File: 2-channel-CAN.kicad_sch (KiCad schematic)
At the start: 21 parts, among them K1 G6K-2 12V, Q1 PZT2222A, U6 MCP2515-xSO, U7 SN65HVD230, U8 SN65HVD230, Y2 8MHz

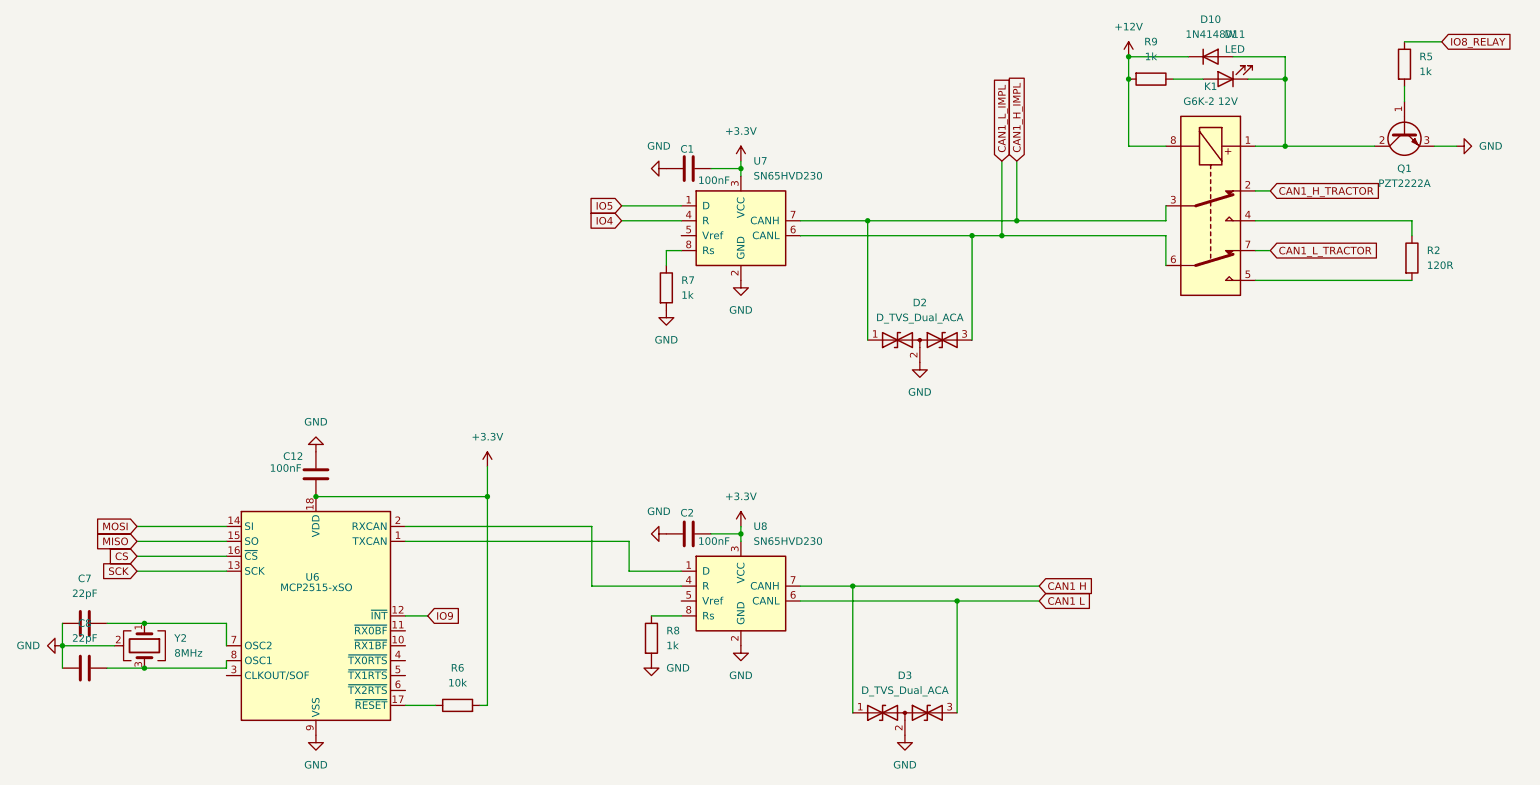
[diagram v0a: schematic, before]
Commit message: Fixes 20/10/2026
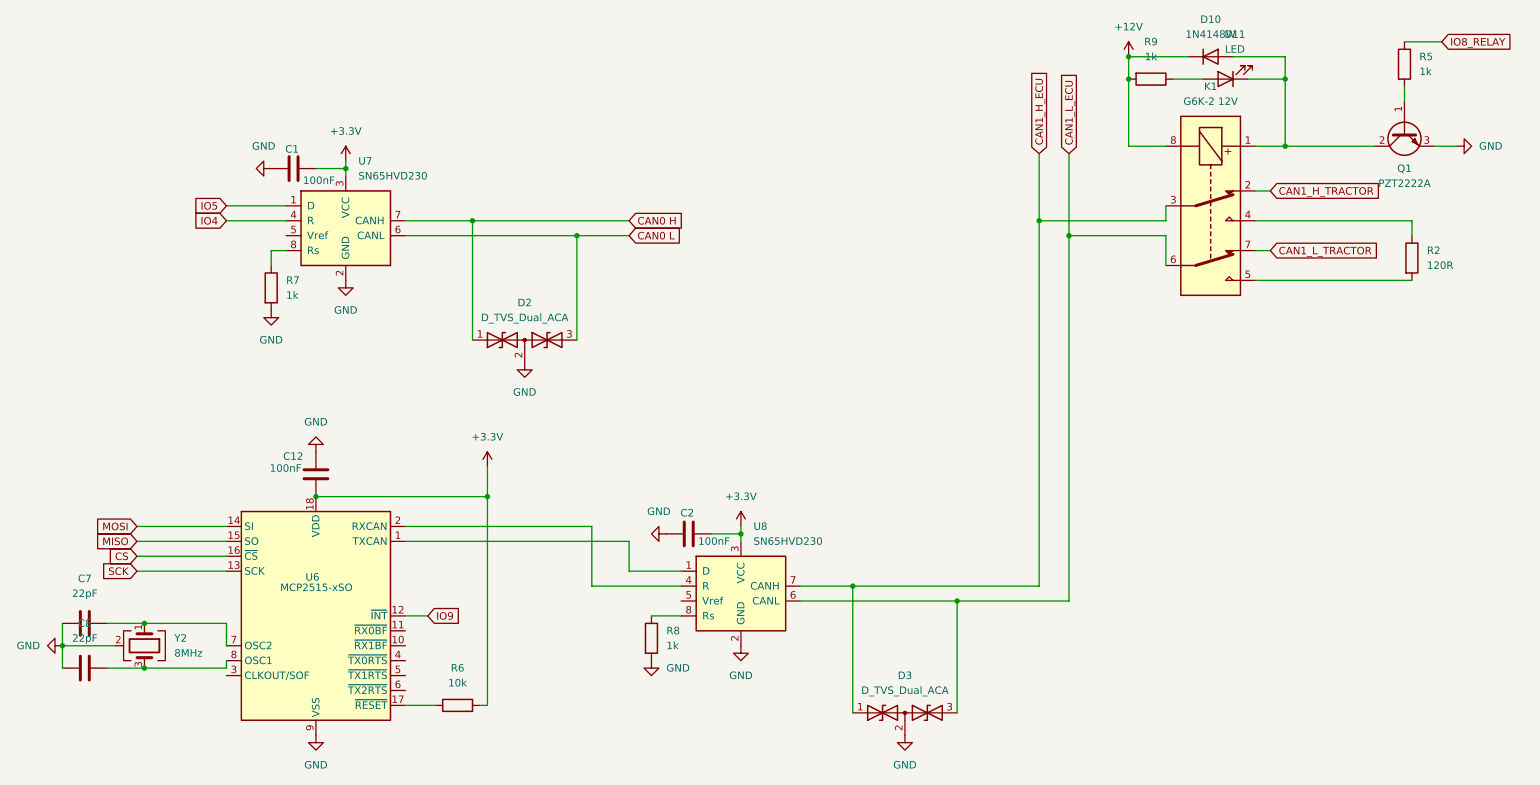
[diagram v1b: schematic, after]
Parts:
- D11: now in the parts list
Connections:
- net CAN1 H renamed CAN1_H_ECU
- net CAN1_H_ECU: now also K1.3
- net CAN1 L renamed CAN1_L_ECU
- net CAN1_L_ECU: now also K1.6
- net CAN1_H_IMPL renamed CAN0 H
- net CAN0 H: no longer K1.3
- net CAN1_L_IMPL renamed CAN0 L
- net CAN0 L: no longer K1.6
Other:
- moved on the sheet: C1, D2, R7, U7
